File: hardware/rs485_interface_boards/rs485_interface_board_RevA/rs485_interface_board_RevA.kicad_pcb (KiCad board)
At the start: 2 copper layers, 19.5 x 42.5 mm, 5 parts, among them J1 615006141121, J3 Conn_01x03, U1 SN65HVD3082EP

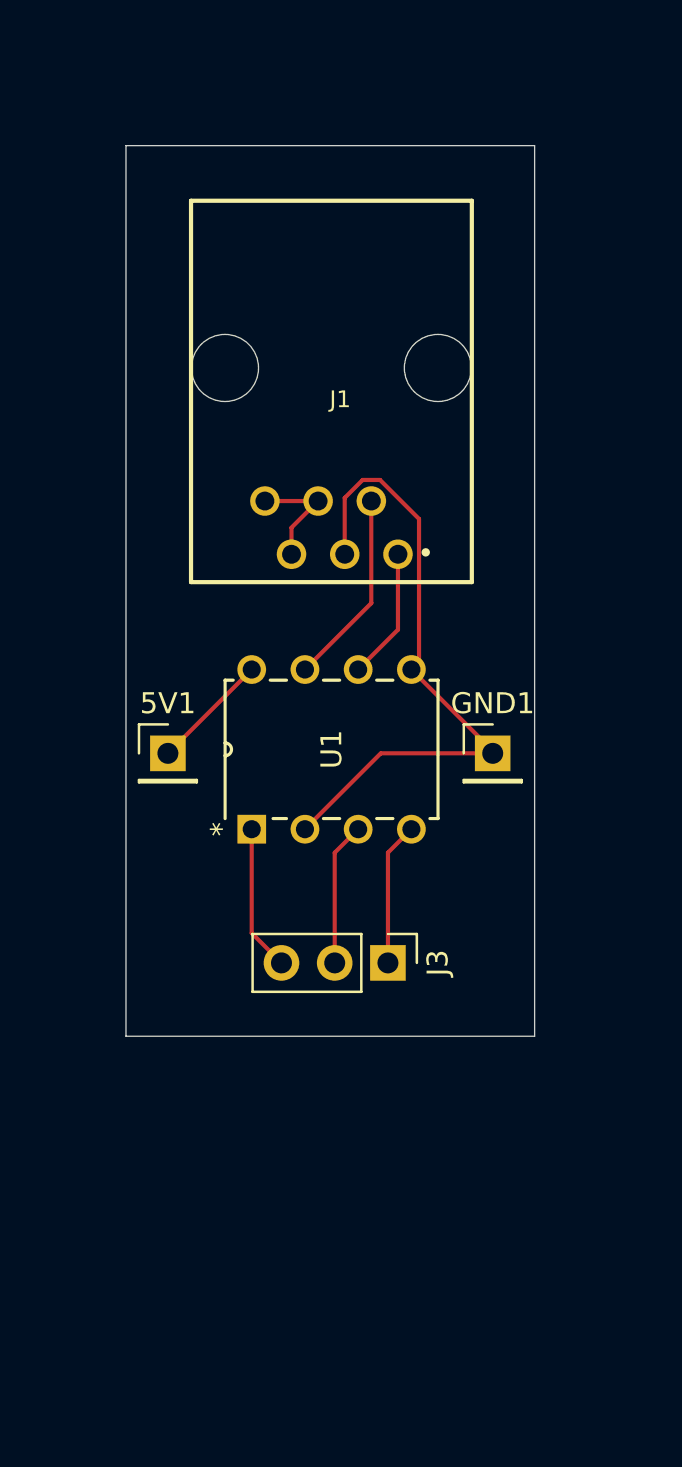
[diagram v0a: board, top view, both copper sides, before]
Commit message: completed rs-485 eth rev a board, generated pcb
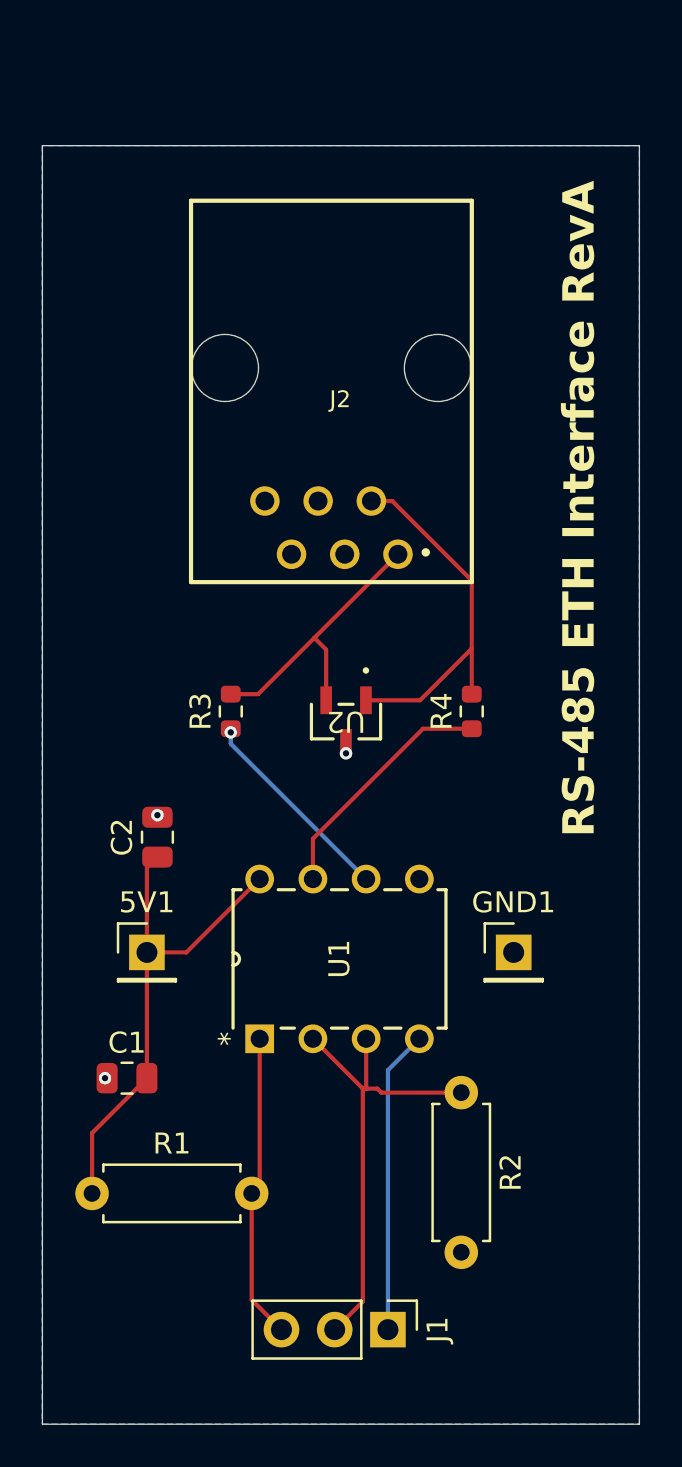
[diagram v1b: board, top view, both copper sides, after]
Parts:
- added C1: 100 nf, Capacitor_SMD:C_0805_2012Metric, F.Cu at (116.5, 114.0)
- added C2: 100 nf, Capacitor_SMD:C_0805_2012Metric, F.Cu at (118.0, 102.5)
- added R1: 10k, Resistor_THT:R_Axial_DIN0207_L6.3mm_D2.5mm_P7.62mm_Horizontal, F.Cu at (114.9, 119.5)
- added R2: 10k, Resistor_THT:R_Axial_DIN0207_L6.3mm_D2.5mm_P7.62mm_Horizontal, F.Cu at (132.5, 114.7)
- added R3: 10 Ohm, Resistor_SMD:R_0603_1608Metric, F.Cu at (121.5, 96.5)
- added R4: 10 Ohm, Resistor_SMD:R_0603_1608Metric, F.Cu at (133.0, 96.5)
- added U2: SM712.TCT, footprints:SOT23_SEM, F.Cu at (127.0, 97.0)
- moved J1 17.5 mm to (129.0, 126.0)
- moved U1 10.0 mm to (126.5, 108.4)
- moved 5V1 9.55 mm to (117.5, 108.0)
- moved GND1 9.55 mm to (135.0, 108.0)
- renumbered J3 to J1, J1 to J2
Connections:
- J1 pad 2: Net-(J3-Pin_2) -> Net-(J1-Pin_2)
- J2 pad 1: Net-(U1-A) -> Net-(J2-Pad1)
- J2 pad 2: Net-(U1-B) -> Net-(J2-Pad2)
- U1 pad 2: GND -> Net-(J1-Pin_2)
- U1 pad 3: Net-(J3-Pin_2) -> Net-(J1-Pin_2)
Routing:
- net GND: track 30.8 -> 0.00 mm, vias 0 -> 3
- net Net-(J1-Pin_2): track 0.00 -> 22.6 mm
- net +5V: track 5.66 -> 24.2 mm
- net Net-(J2-Pad2): track 0.00 -> 17.9 mm
- net Net-(J2-Pad1): track 0.00 -> 14.0 mm
- net Net-(J1-Pin_3): track 6.97 -> 15.0 mm
- net Net-(J1-Pin_1): track 7.08 -> 14.5 mm
- net Net-(J3-Pin_2): track 6.84 -> 0.00 mm
- net unconnected-(J2-Pad4): track 5.61 -> 0.00 mm
- net Net-(U1-A): track 6.29 -> 9.68 mm, vias 0 -> 1
- net Net-(U1-B): track 9.35 -> 11.7 mm
- added copper zone on B.Cu, net GND
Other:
- board size 19.5 x 42.5 mm -> 28.5 x 61 mm
- board text added: "RS-485 ETH Interface RevA"
